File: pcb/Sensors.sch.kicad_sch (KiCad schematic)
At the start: 22 parts, among them J1 53398-0371, J2 53398-0371, J3 Conn_01x04_Pin, J4 53398-0371, J5 53398-0371, J6 53398-0371, J7 53398-0371, J8 53398-0371, J9 53398-0371, U2 BMP280

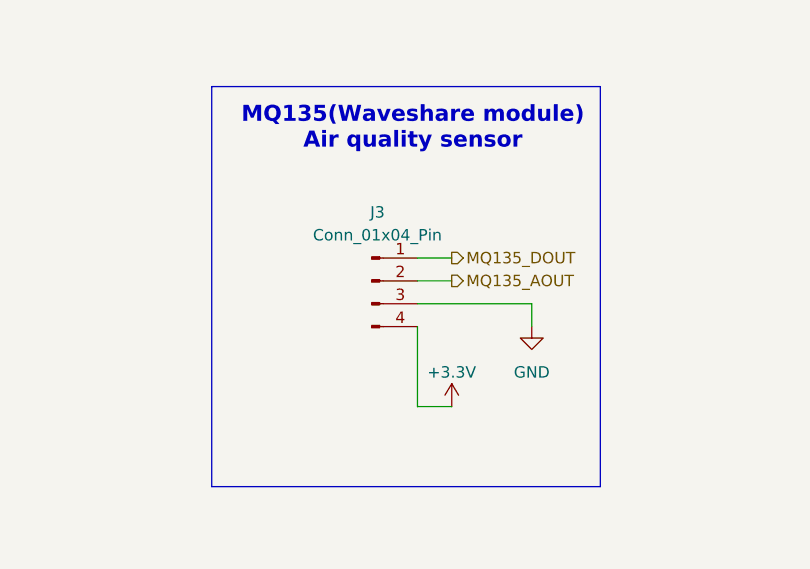
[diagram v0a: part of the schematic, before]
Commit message: Drobne poprawki w schemacie elektrycznym
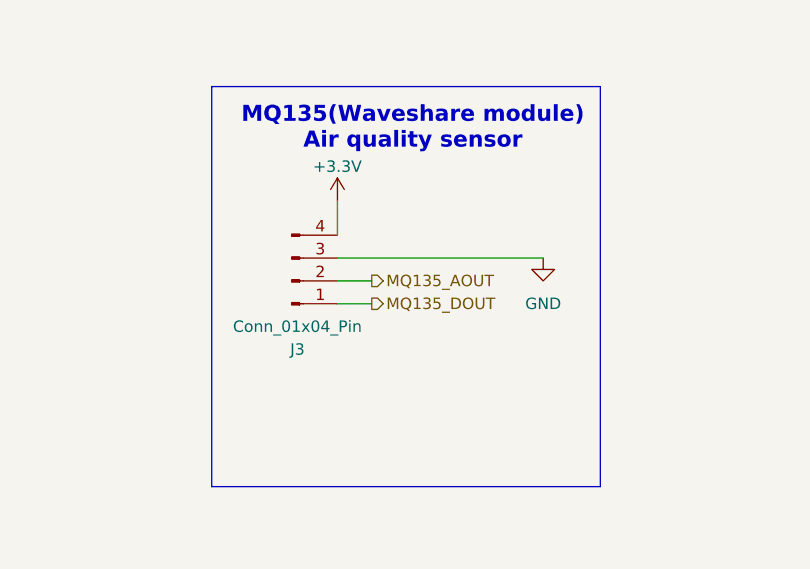
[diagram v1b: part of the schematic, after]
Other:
- moved on the sheet: J3
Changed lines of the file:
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@@
 	(wire
 		(pts
-			(xy 198.12 72.39) (xy 198.12 69.85)
+			(xy 121.92 85.09) (xy 121.92 100.33)
 		)
 		(stroke
@@
 	(wire
 		(pts
-			(xy 121.92 85.09) (xy 121.92 100.33)
+			(xy 106.68 116.84) (xy 106.68 118.11)
 		)
 		(stroke
@@
 	(wire
 		(pts
-			(xy 106.68 116.84) (xy 106.68 118.11)
+			(xy 86.36 171.45) (xy 91.44 171.45)
 		)
 		(stroke
@@
 	(wire
 		(pts
-			(xy 86.36 171.45) (xy 91.44 171.45)
+			(xy 86.36 173.99) (xy 91.44 173.99)
 		)
 		(stroke
@@
 	(wire
 		(pts
-			(xy 86.36 173.99) (xy 91.44 173.99)
+			(xy 167.64 124.46) (xy 167.64 125.73)
 		)
 		(stroke
@@
 	(wire
 		(pts
-			(xy 167.64 124.46) (xy 167.64 125.73)
+			(xy 105.41 45.72) (xy 102.87 45.72)
 		)
 		(stroke
@@
 	(wire
 		(pts
-			(xy 105.41 45.72) (xy 102.87 45.72)
+			(xy 109.22 116.84) (xy 121.92 116.84)
 		)
 		(stroke
@@
 	(wire
 		(pts
-			(xy 109.22 116.84) (xy 121.92 116.84)
+			(xy 176.53 58.42) (xy 176.53 62.23)
 		)
 		(stroke
@@
 	(wire
 		(pts
+			(xy 176.53 67.31) (xy 180.34 67.31)
+		)
+		(stroke
+			(width 0)
+			(type default)
+		)
+	)
+	(wire
+		(pts
 			(xy 104.14 118.11) (xy 104.14 116.84)
 		)
@@
 	(wire
 		(pts
-			(xy 185.42 81.28) (xy 189.23 81.28)
-		)
-		(stroke
-			(width 0)
-			(type default)
-		)
-	)
-	(wire
-		(pts
 			(xy 121.92 50.8) (xy 123.19 50.8)
 		)
@@
 	(wire
 		(pts
-			(xy 198.12 69.85) (xy 185.42 69.85)
-		)
-		(stroke
-			(width 0)
-			(type default)
-		)
-	)
-	(wire
-		(pts
 			(xy 76.2 102.87) (xy 77.47 102.87)
 		)
@@
 	(wire
 		(pts
-			(xy 185.42 72.39) (xy 185.42 81.28)
-		)
-		(stroke
-			(width 0)
-			(type default)
-		)
-	)
-	(wire
-		(pts
 			(xy 78.74 106.68) (xy 77.47 106.68)
 		)
@@
 	(wire
 		(pts
-			(xy 185.42 64.77) (xy 189.23 64.77)
-		)
-		(stroke
-			(width 0)
-			(type default)
-		)
-	)
-	(wire
-		(pts
 			(xy 104.14 184.15) (xy 104.14 186.69)
 		)
@@
 	(wire
 		(pts
-			(xy 185.42 67.31) (xy 189.23 67.31)
+			(xy 123.19 48.26) (xy 123.19 50.8)
 		)
 		(stroke
@@
 	(wire
 		(pts
-			(xy 123.19 48.26) (xy 123.19 50.8)
+			(xy 176.53 69.85) (xy 180.34 69.85)
 		)
 		(stroke
@@
 	(wire
 		(pts
+			(xy 176.53 64.77) (xy 199.39 64.77)
+		)
+		(stroke
+			(width 0)
+			(type default)
+		)
+	)
+	(wire
+		(pts
 			(xy 73.66 160.02) (xy 73.66 179.07)
 		)
@@
 	(hierarchical_label "MQ135_AOUT"
 		(shape output)
-		(at 189.23 67.31 0)
+		(at 180.34 67.31 0)
 		(fields_autoplaced yes)
 		(effects
@@
 	(hierarchical_label "MQ135_DOUT"
 		(shape output)
-		(at 189.23 64.77 0)
+		(at 180.34 69.85 0)
 		(fields_autoplaced yes)
 		(effects
@@
 	(symbol
 		(lib_id "power:+3.3V")
-		(at 189.23 81.28 0)
+		(at 176.53 58.42 0)
 		(unit 1)
 		(exclude_from_sim no)
@@
 		(dnp no)
 		(property "Reference" "#PWR021"
-			(at 189.23 85.09 0)
+			(at 176.53 62.23 0)
 			(effects
 				(font
@@
 		)
 		(property "Value" "+3.3V"
-			(at 189.23 77.47 0)
+			(at 176.53 54.61 0)
 			(effects
 				(font
@@
 		)
 		(property "Footprint" ""
-			(at 189.23 81.28 0)
+			(at 176.53 58.42 0)
 			(effects
 				(font
@@
 		)
 		(property "Datasheet" ""
-			(at 189.23 81.28 0)
+			(at 176.53 58.42 0)
 			(effects
 				(font
@@
 		)
 		(property "Description" "Power symbol creates a global label with name \"+3.3V\""
-			(at 189.23 81.28 0)
+			(at 176.53 58.42 0)
 			(effects
 				(font
@@
 	(symbol
 		(lib_id "Connector:Conn_01x04_Pin")
-		(at 180.34 67.31 0)
+		(at 171.45 67.31 0)
+		(mirror x)
 		(unit 1)
 		(exclude_from_sim no)
@@
 		(on_board yes)
 		(dnp no)
-		(fields_autoplaced yes)
 		(property "Reference" "J3"
-			(at 180.975 59.69 0)
+			(at 172.085 74.93 0)
 			(effects
 				(font
@@
 		)
 		(property "Value" "Conn_01x04_Pin"
-			(at 180.975 62.23 0)
+			(at 172.085 72.39 0)
 			(effects
 				(font
@@
 		)
 		(property "Footprint" "1bmoje:533980471- MOLEXx4"
-			(at 180.34 67.31 0)
+			(at 171.45 67.31 0)
 			(effects
 				(font
@@
 		)
 		(property "Datasheet" "~"
-			(at 180.34 67.31 0)
+			(at 171.45 67.31 0)
 			(effects
 				(font
@@
 		)
 		(property "Description" "Generic connector, single row, 01x04, script generated"
-			(at 180.34 67.31 0)
+			(at 171.45 67.31 0)
 			(effects
 				(font
@@
 	(symbol
 		(lib_id "power:GND")
-		(at 198.12 72.39 0)
+		(at 199.39 64.77 0)
 		(unit 1)
 		(exclude_from_sim no)
@@
 		(fields_autoplaced yes)
 		(property "Reference" "#PWR022"
-			(at 198.12 78.74 0)
+			(at 199.39 71.12 0)
 			(effects
 				(font
@@
 		)
 		(property "Value" "GND"
-			(at 198.12 77.47 0)
+			(at 199.39 69.85 0)
 			(effects
 				(font
@@
 		)
 		(property "Footprint" ""
-			(at 198.12 72.39 0)
+			(at 199.39 64.77 0)
 			(effects
 				(font
@@
 		)
 		(property "Datasheet" ""
-			(at 198.12 72.39 0)
+			(at 199.39 64.77 0)
 			(effects
 				(font
@@
 		)
 		(property "Description" "Power symbol creates a global label with name \"GND\" , ground"
-			(at 198.12 72.39 0)
+			(at 199.39 64.77 0)
 			(effects
 				(font
